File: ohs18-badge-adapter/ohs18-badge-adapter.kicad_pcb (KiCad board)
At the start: 2 copper layers, 4 parts, among them J1 OHS18 badge J1, J2 FTDI 3.3V USB to Serial

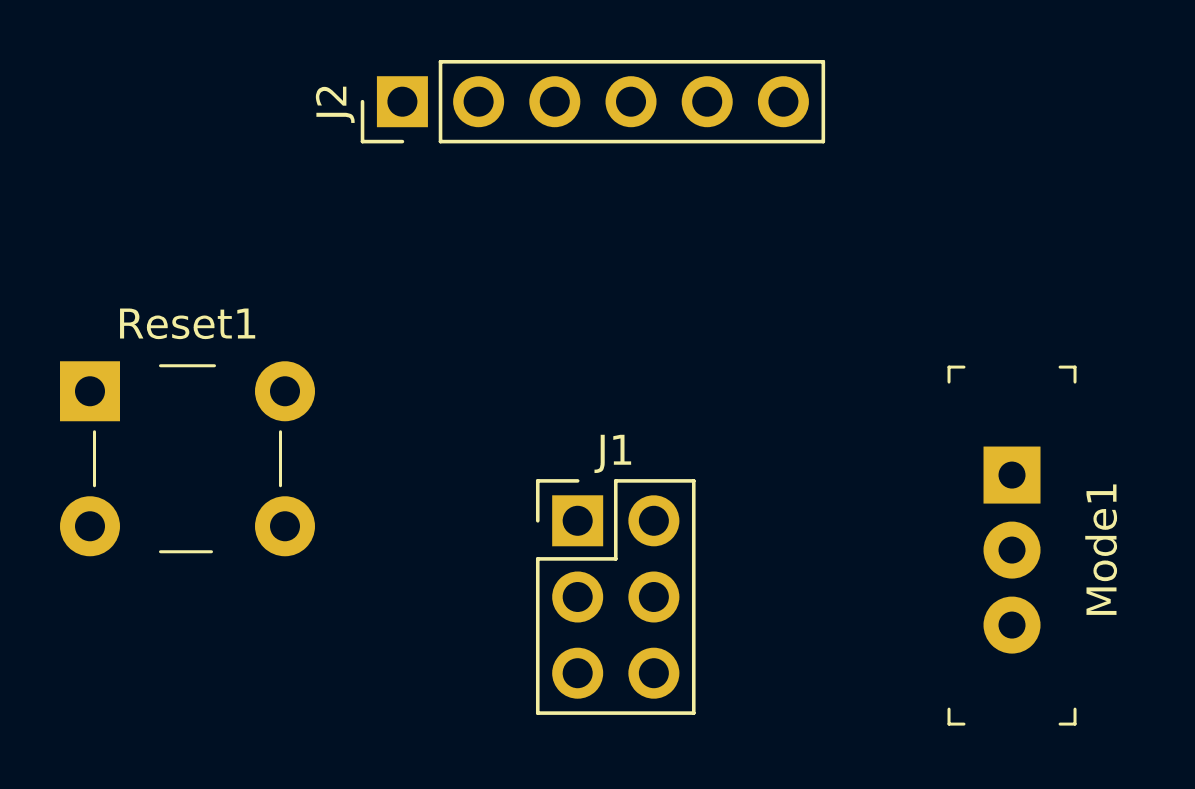
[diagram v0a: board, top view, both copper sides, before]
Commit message: finish layout of rev 1
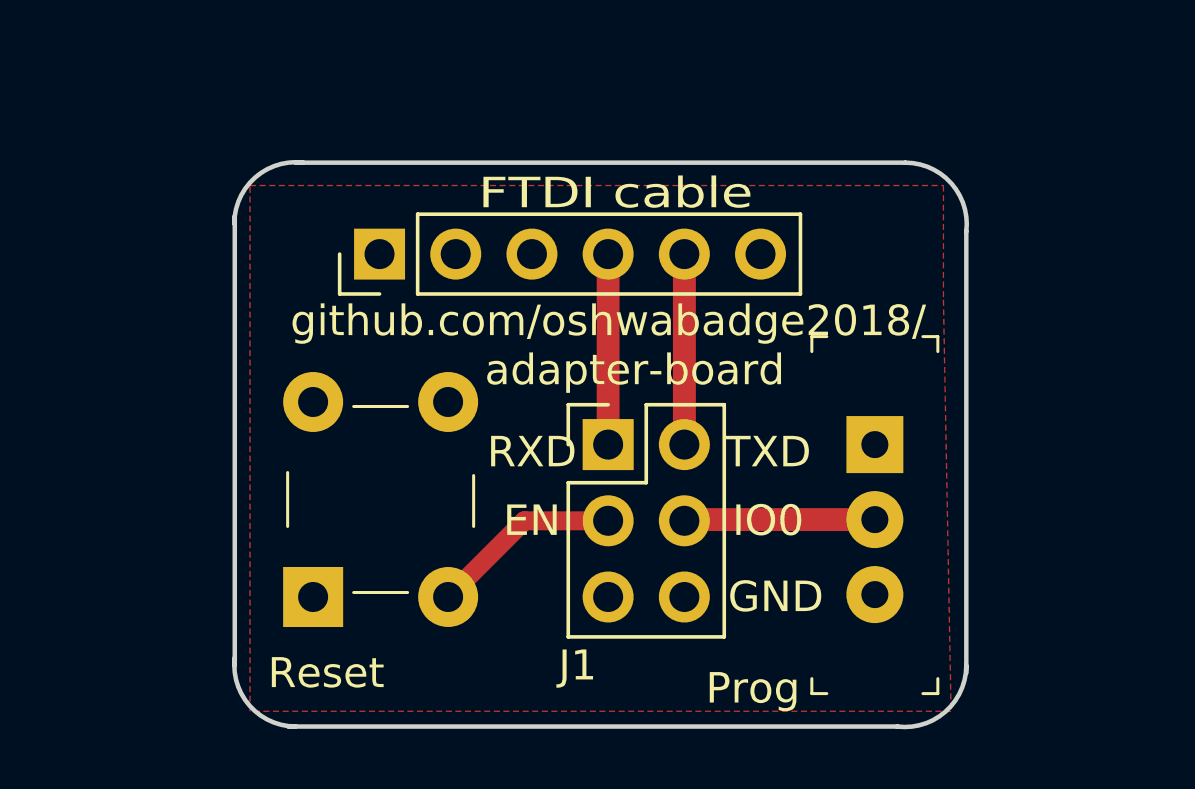
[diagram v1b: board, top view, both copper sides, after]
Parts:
- removed Reset1: B3F-1000, digikey-footprints:Switch_Tactile_THT_B3F-1xxx
- added Reset: B3F-1000, digikey-footprints:Switch_Tactile_THT_B3F-1xxx, F.Cu at (131.4, 83.6)
- J1: value OHS18 badge J1 -> OHS18 Badge
- moved J2 5.14 mm to (133.6, 72.1)
- moved Mode1 4.68 mm to (150.1, 78.5)
- moved J1 2.74 mm to (141.2, 78.5)
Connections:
- J1 pad 2: EN -> RXD
- J1 pad 3: Net-(J1-Pad3) -> EN
- J1 pad 4: RXD -> IO0
- J1 pad 5: IO0 -> Net-(J1-Pad5)
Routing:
- net EN: track 0.00 -> 6.39 mm
- net IO0: track 0.00 -> 6.37 mm
- net TXD: track 0.00 -> 6.35 mm
- net RXD: track 0.00 -> 6.35 mm
- added copper zone on F.Cu, net GND
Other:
- board outline added: 24.4 x 18.8 mm
- net class Default: clearance 0.2 -> 0.508; trace_width 0.25 -> 0.508; via_drill 0.4 -> 0.508
- rule trace_clearance: 0.2 -> 0.508
- rule trace_min: 0.2 -> 0.254
- rule via_min_drill: 0.3 -> 0.508
- rule via_min_size: 0.4 -> 0.381
- board text added: "#ohsummit18"
- board text added: "EN"
- board text added: "FTDI cable"
- board text added: "GND"
- board text added: "IO0"
- board text added: "Prog"
- board text added: "RXD"
- board text added: "TXD"
- board text added: "drew@oshpark.com"
- board text added: "github.com/oshwabadge2018/ adapter-board"
